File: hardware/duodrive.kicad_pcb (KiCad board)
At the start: 2 copper layers, 49 x 75 mm, 105 parts, among them J1 Power, J10 Power, J2 Conn_02x08_Odd_Even, J3 Conn_01x03, J7 Conn_01x04, J8 Conn_01x04, J9 Power, Q1 AOD4184, Q2 AOD4184, Q3 AOD4184, Q4 AOD4184, Q5 AOD4184, Q6 AOD4184, Q7 AOD4184, Q8 AOD4184, U10 MIC5219-3.3YM5, U2 IR2011, U3 TPS62173DSG, U4 STM32G431RBTx, U5 IR2011, U6 IR2011, U7 IR2011, U8 TPS62933, U9 TJA1042T, Y1 Resonator

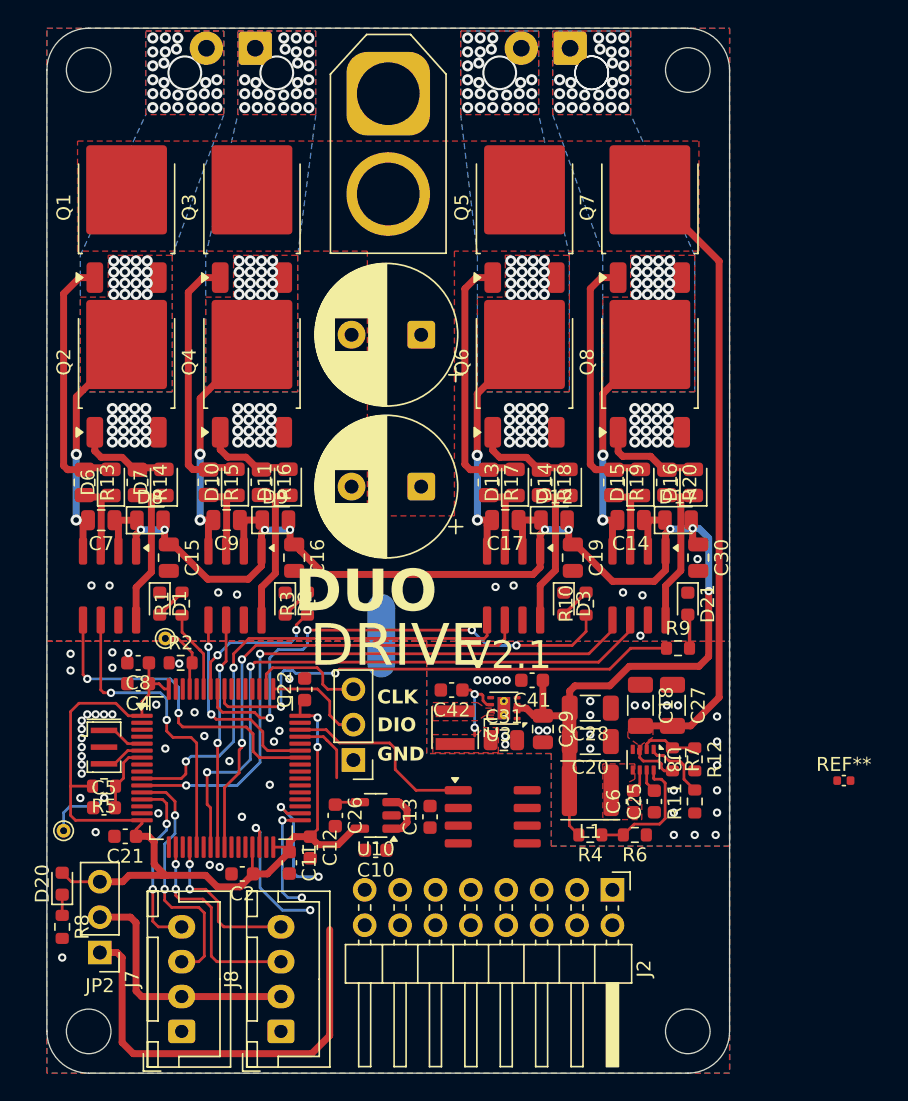
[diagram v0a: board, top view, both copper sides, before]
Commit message: test
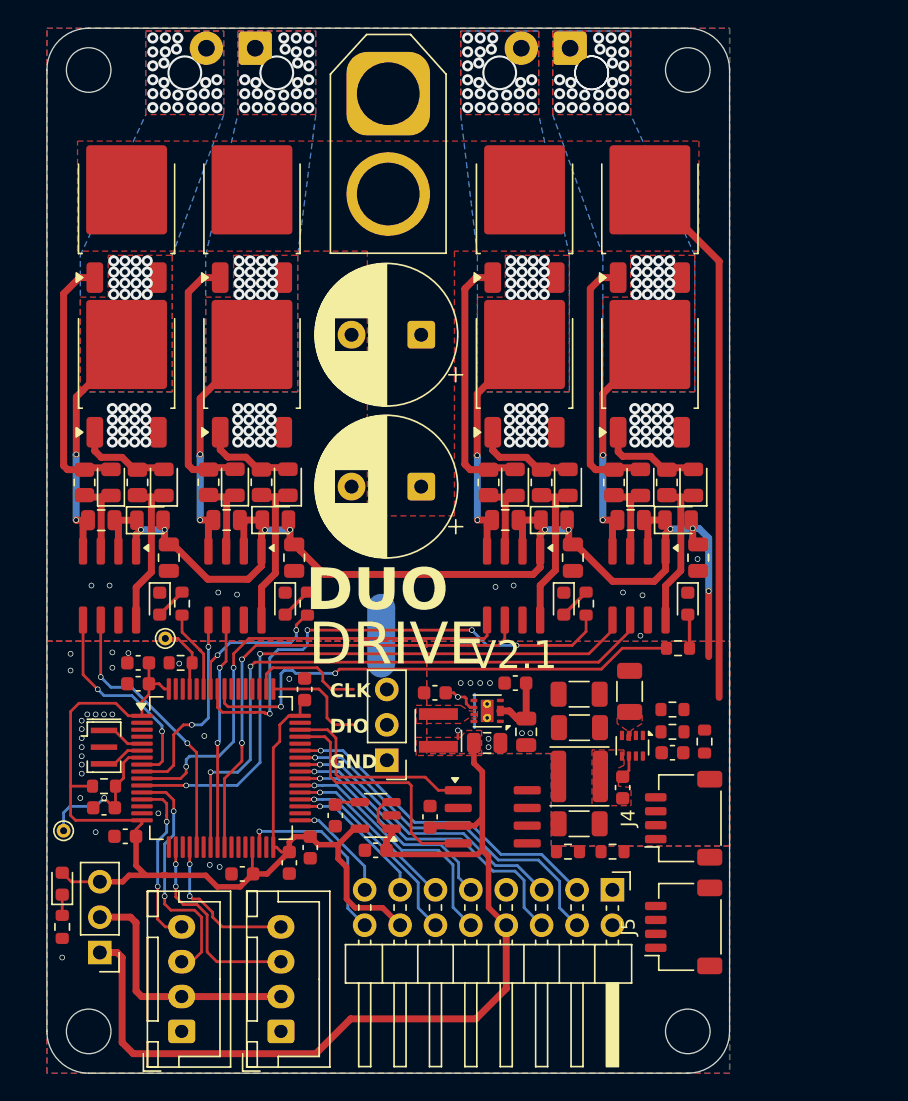
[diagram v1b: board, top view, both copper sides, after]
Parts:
- removed REF**: C_0402_1005Metric, Capacitor_SMD:C_0402_1005Metric
- added J4: Conn_01x04, Connector_JST:JST_SH_SM04B-SRSS-TB_1x04-1MP_P1.00mm_Horizontal, F.Cu at (135.7, 106.7)
- added J5: Conn_01x04, Connector_JST:JST_SH_SM04B-SRSS-TB_1x04-1MP_P1.00mm_Horizontal, F.Cu at (135.7, 114.5)
- moved C28 8.34 mm to (128.2, 107.1)
- moved C27 6.75 mm to (128.2, 97.8), turned to 0 degrees
- moved R11 5.25 mm to (134.9, 100.5), turned to 180 degrees
- moved C25 3.73 mm to (134.9, 102.0), turned to 180 degrees
- moved R7 3.57 mm to (134.9, 98.9), turned to 180 degrees
- moved J3 2.40 mm to (114.4, 102.5)
- moved R4 2.00 mm to (127.4, 109.1)
- moved R6 2.00 mm to (130.6, 109.1)
- moved R12 1.45 mm to (137.2, 101.2)
- moved C18 1.27 mm to (131.8, 97.6)
- moved C20 1.27 mm to (128.2, 100.2)
- moved C6 1.27 mm to (131.3, 104.5)
- moved L1 1.27 mm to (128.2, 103.7)
- moved U8 1.27 mm to (132.0, 101.5)
- moved C31 1.22 mm to (121.6, 101.3)
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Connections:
- J2 pad 1: unconnected-(J2-Pin_1-Pad1) -> GNDS
- J2 pad 10: unconnected-(J2-Pin_10-Pad10) -> PC6
- J2 pad 11: unconnected-(J2-Pin_11-Pad11) -> SPI_MOSI
- J2 pad 12: unconnected-(J2-Pin_12-Pad12) -> SPI_MISO
- J2 pad 13: unconnected-(J2-Pin_13-Pad13) -> SPI_CLK
- J2 pad 14: unconnected-(J2-Pin_14-Pad14) -> +3.3V
- J2 pad 15: unconnected-(J2-Pin_15-Pad15) -> RX
- J2 pad 16: unconnected-(J2-Pin_16-Pad16) -> TX
- J2 pad 3: unconnected-(J2-Pin_3-Pad3) -> PA9
- J2 pad 4: unconnected-(J2-Pin_4-Pad4) -> PA8
- J2 pad 5: unconnected-(J2-Pin_5-Pad5) -> PC9
- J2 pad 6: unconnected-(J2-Pin_6-Pad6) -> PC8
- J2 pad 7: unconnected-(J2-Pin_7-Pad7) -> GNDS
- J2 pad 8: unconnected-(J2-Pin_8-Pad8) -> +5V
- J2 pad 9: unconnected-(J2-Pin_9-Pad9) -> PC7
- U4 pad 35: unconnected-(U4-PB13-Pad35) -> SPI_CLK
- U4 pad 36: unconnected-(U4-PB14-Pad36) -> SPI_MISO
- U4 pad 37: unconnected-(U4-PB15-Pad37) -> SPI_MOSI
- U4 pad 38: unconnected-(U4-PC6-Pad38) -> PC6
- U4 pad 39: unconnected-(U4-PC7-Pad39) -> PC7
- U4 pad 40: unconnected-(U4-PC8-Pad40) -> PC8
- U4 pad 41: unconnected-(U4-PC9-Pad41) -> PC9
- U4 pad 42: H1 -> PA8
- U4 pad 43: H2 -> PA9
- U4 pad 8: unconnected-(U4-PC0-Pad8) -> H1
- U4 pad 9: unconnected-(U4-PC1-Pad9) -> H2
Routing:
- net +5V: track 40.5 -> 78.1 mm
- net PA8: track 0.00 -> 26.0 mm, vias 0 -> 1
- net PA9: track 0.00 -> 24.0 mm, vias 0 -> 1
- net +10V: track 97.4 -> 74.2 mm
- net PC8: track 0.00 -> 23.1 mm, vias 0 -> 1
- net PC9: track 0.00 -> 21.2 mm, vias 0 -> 1
- net PC6: track 0.00 -> 18.2 mm, vias 0 -> 1
- net PC7: track 0.00 -> 16.2 mm, vias 0 -> 1
- net SPI_MISO: track 0.00 -> 14.5 mm, vias 0 -> 1
- net CANRX: track 5.02 -> 18.0 mm
- net SPI_MOSI: track 0.00 -> 12.6 mm, vias 0 -> 1
- net SPI_CLK: track 0.00 -> 10.4 mm, vias 0 -> 1
- net VDC: track 46.2 -> 36.2 mm
- net Net-(U8-FB): track 9.16 -> 0.00 mm
- net H1: track 24.2 -> 15.2 mm
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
